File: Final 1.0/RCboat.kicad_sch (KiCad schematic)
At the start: 45 parts, among them J1 Conn_02x10_Odd_Even, J2 Battery, J3 Battery, M1 Motor_Servo, M2 Motor_Servo, SW1 SW_Push, SW2 SW_SPDT, U1 BD9G341EFJ, U2 AMS1117-3.3, U3 NRF24L01_Breakout, U4 STM32F100C4Tx, U5 MPU-6000, Y1 8.000MHZ

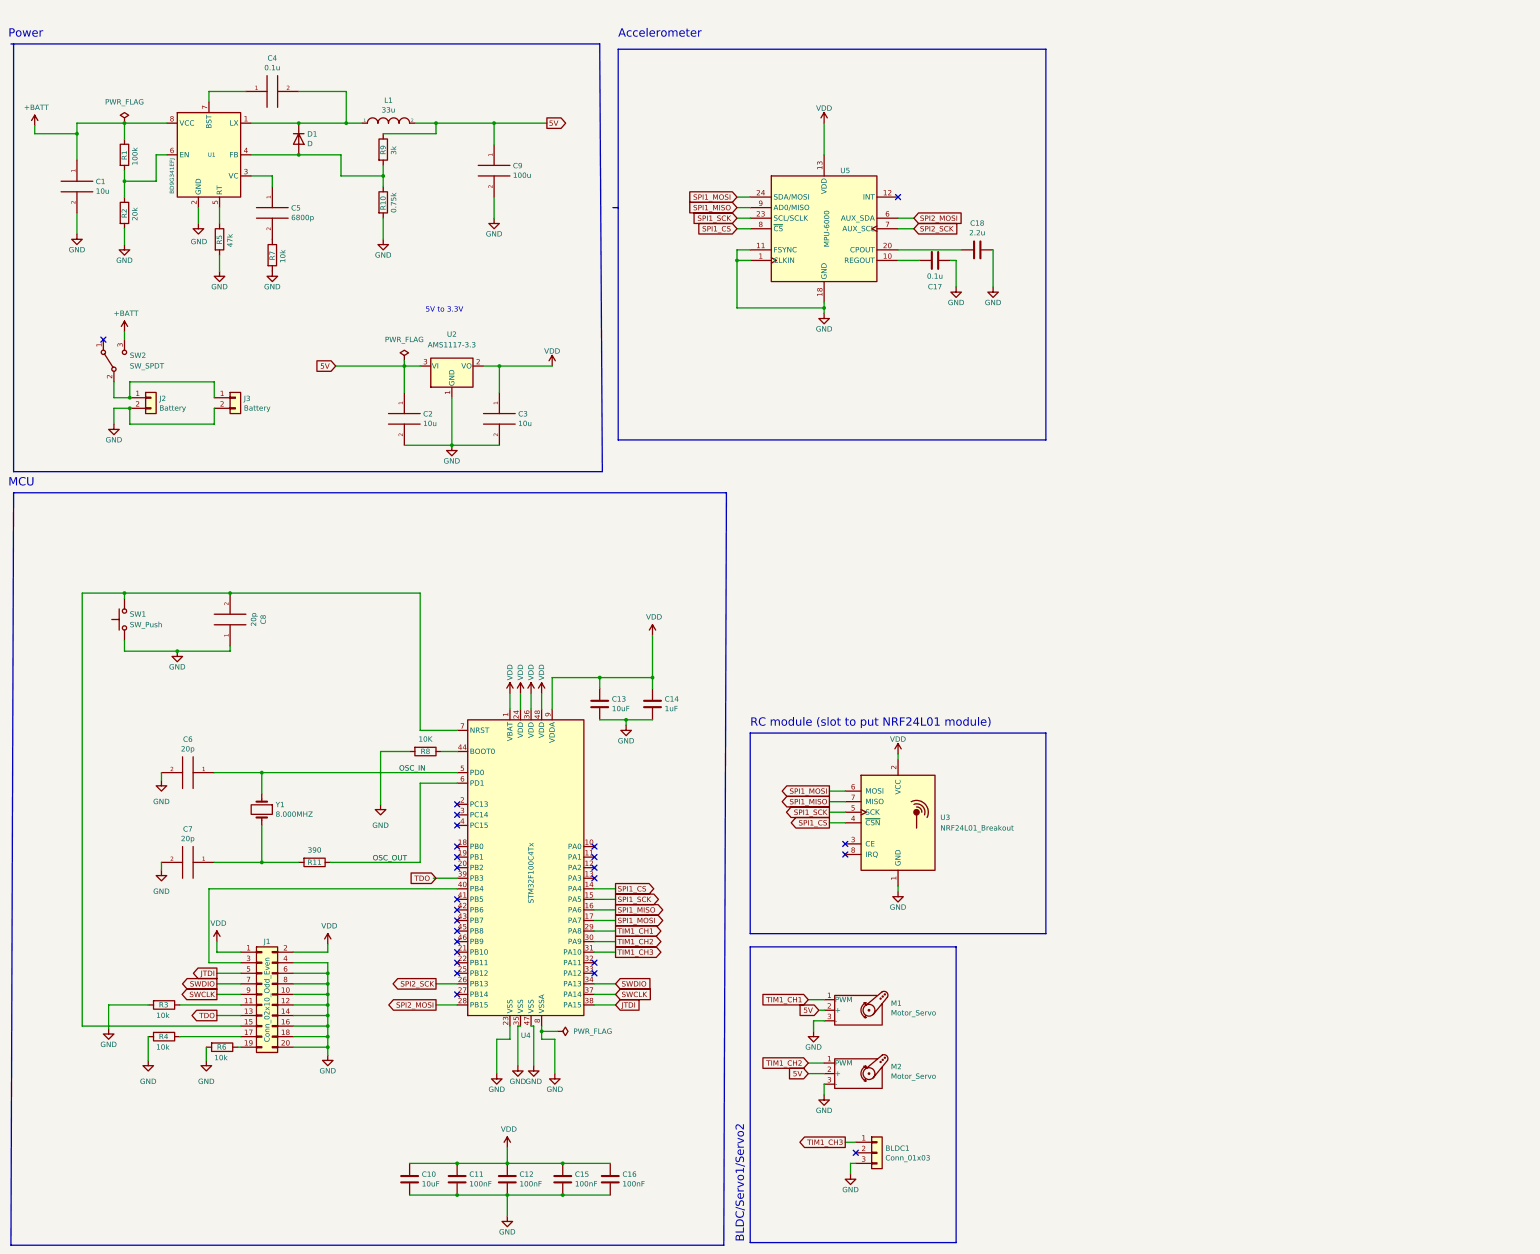
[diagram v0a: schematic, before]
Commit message: Add files via upload
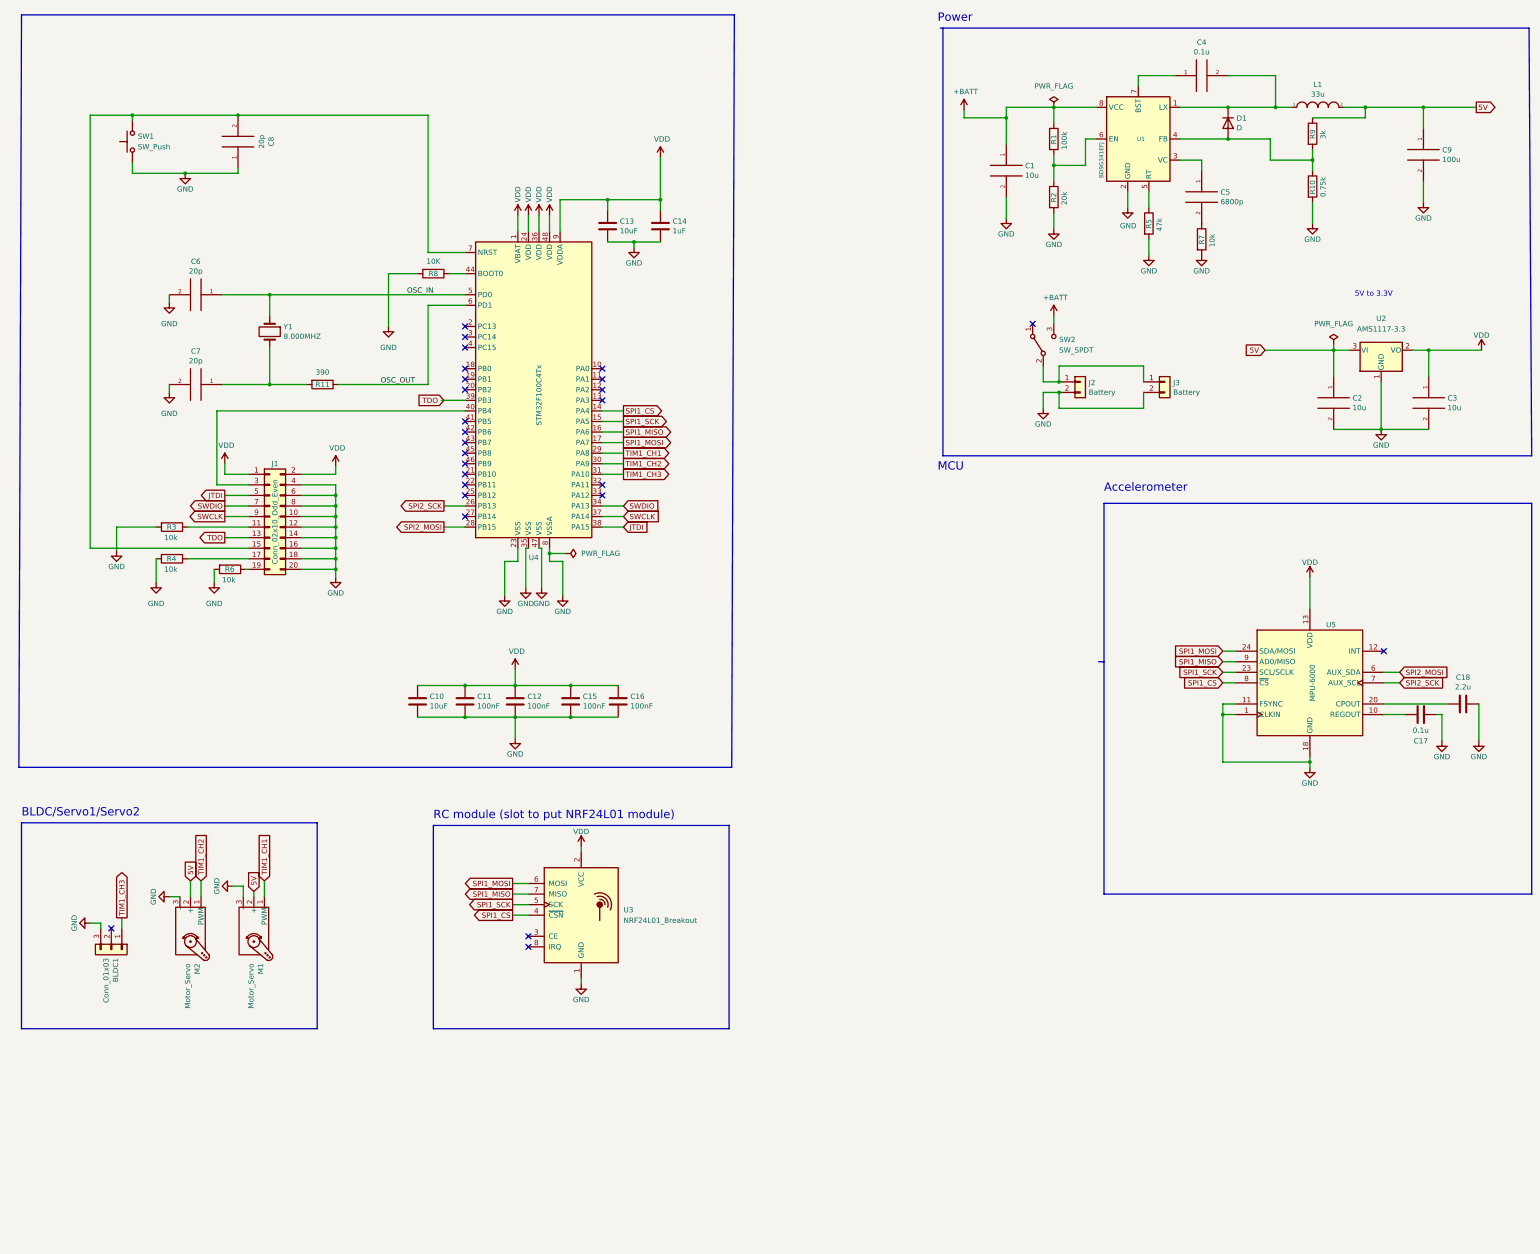
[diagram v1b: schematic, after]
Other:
- moved on the sheet: BLDC1, C1, C10, C11, C12, C13, C14, C15, C16, C17, C18, C2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
